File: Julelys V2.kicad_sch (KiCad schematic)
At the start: 16 parts, among them U2 74HC4051

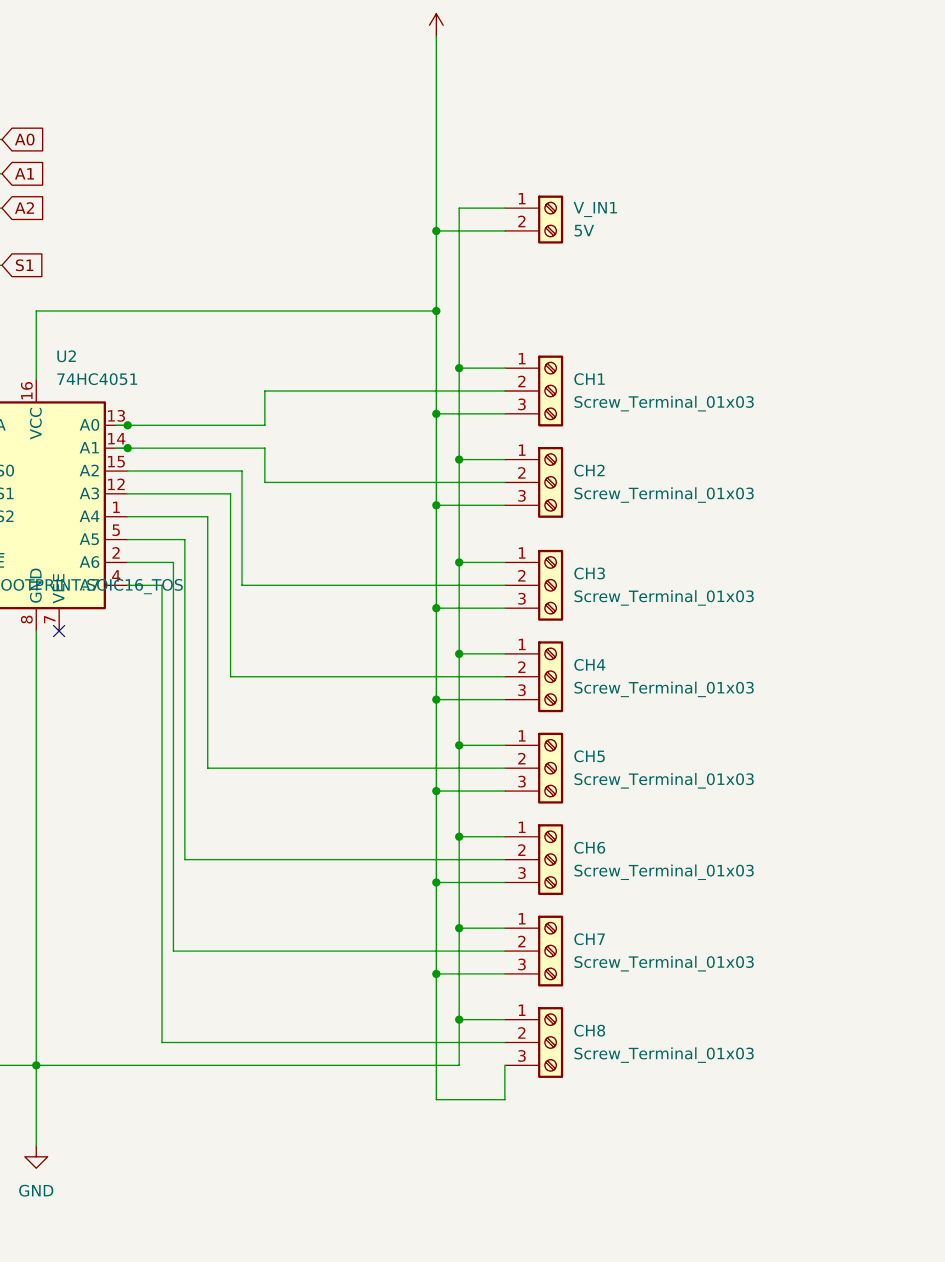
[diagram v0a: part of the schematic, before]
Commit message: Update to V2.1
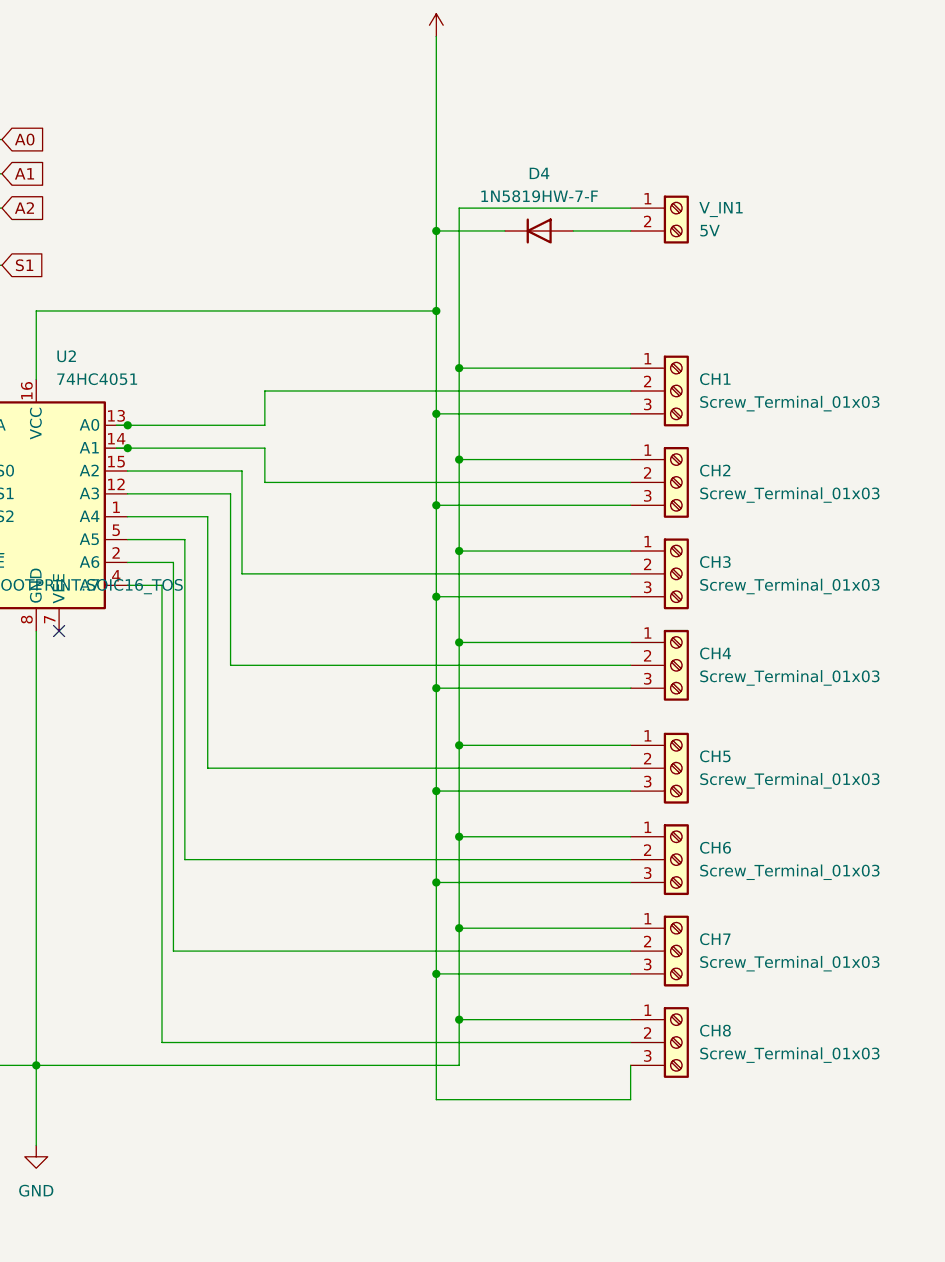
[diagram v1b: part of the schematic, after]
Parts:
- added D4: 1N5819HW-7-F, Diode_SMD:D_SOD-123, symbol Device:D
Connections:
- net +5V: now also D4.1 (K); no longer V_IN1.2 (Pin_2)
- new net: D4.2 (A), V_IN1.2 (Pin_2)
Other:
- moved on the sheet: CH1, CH2, CH3, CH4, CH5, CH6, CH7, CH8, V_IN1
